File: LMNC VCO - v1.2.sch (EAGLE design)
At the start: 79 parts, among them IC1 CEM3340, J1 JACKS, J10 LINK, J13 OCT SEL, P1 POWER, U1 TL072CP, U2 TL074CN, U4 LM4040AIZ, U5 L7805

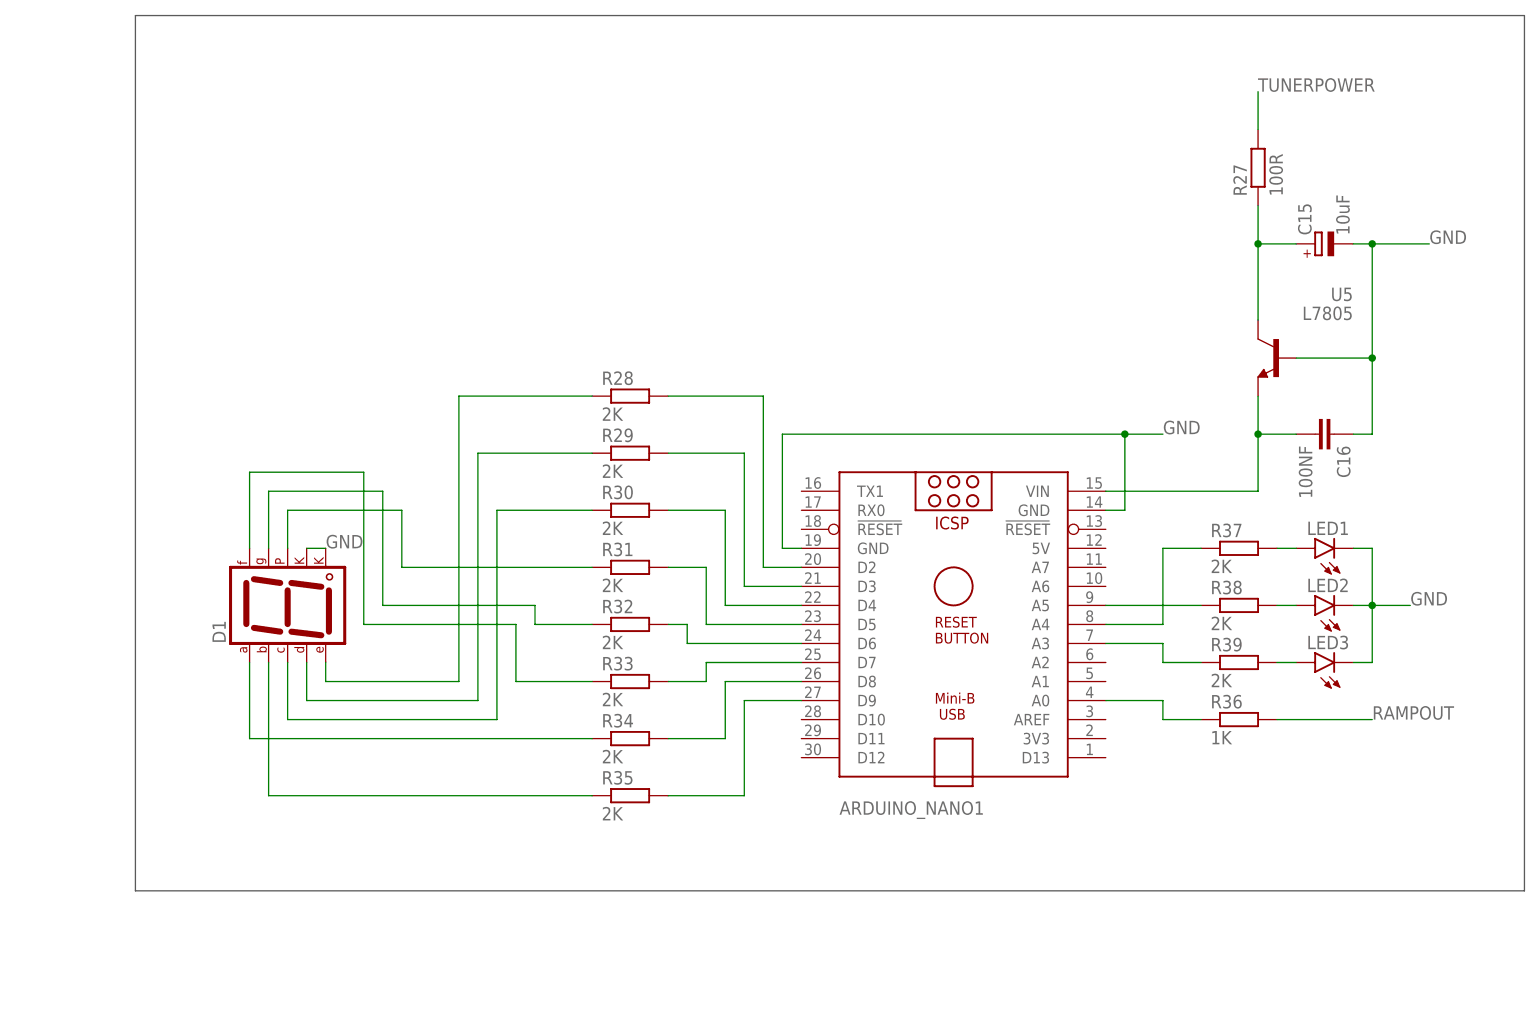
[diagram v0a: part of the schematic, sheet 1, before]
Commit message: Update1
Removed Tuner Arduino,
Replaced Caps to SMD footprint
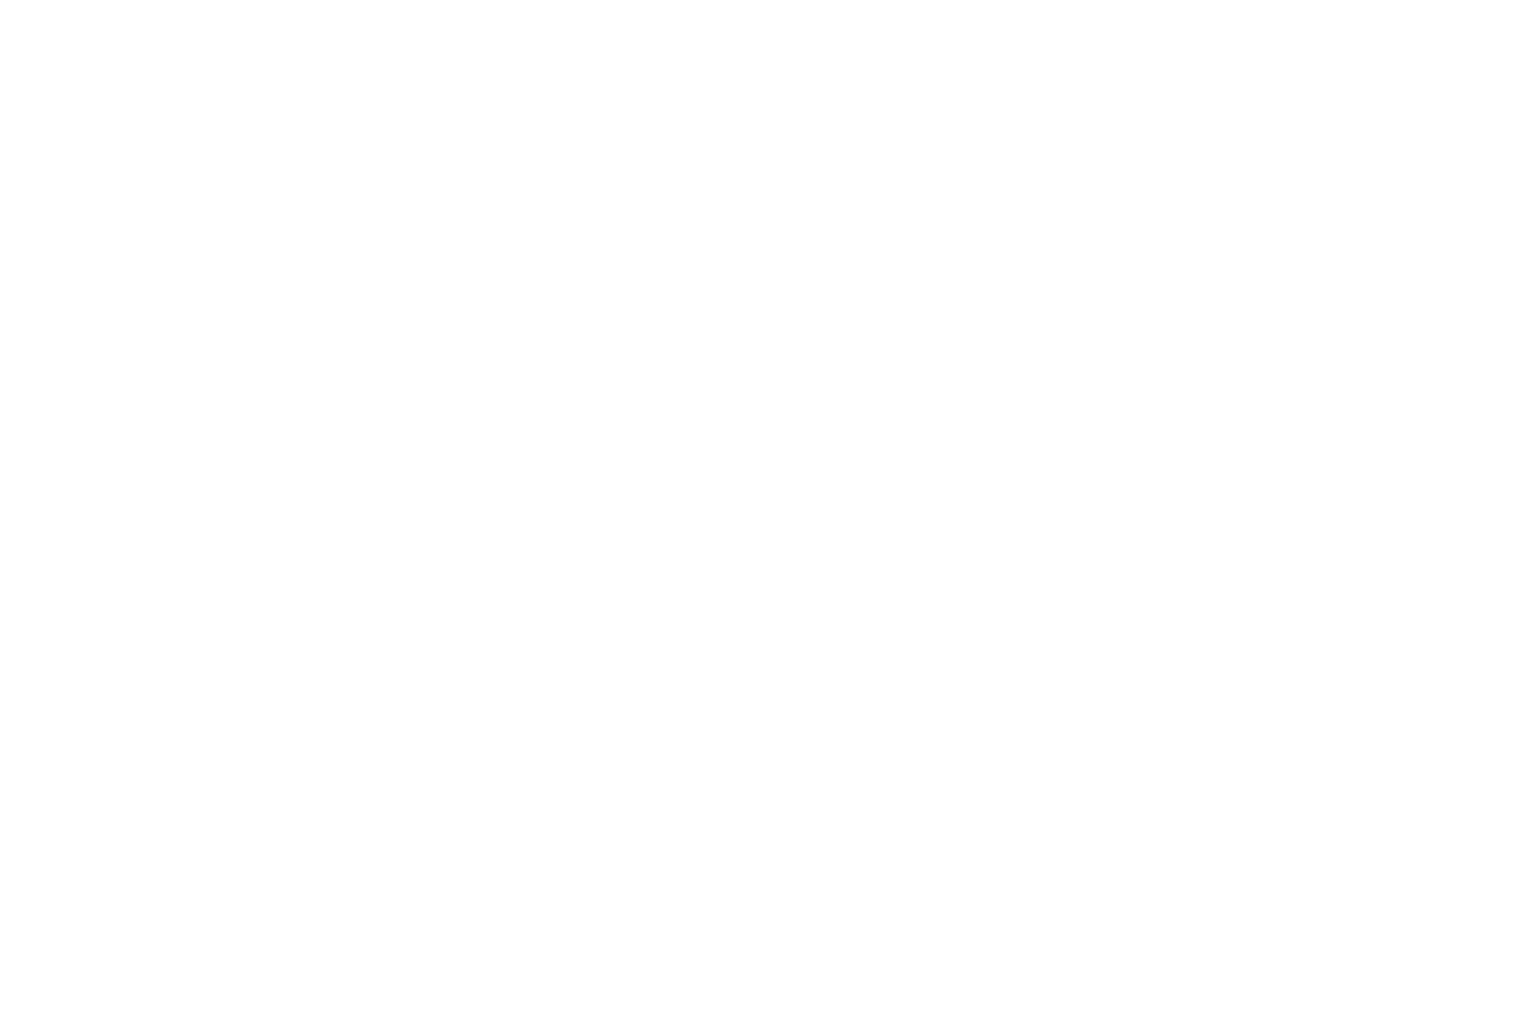
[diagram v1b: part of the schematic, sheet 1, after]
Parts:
- removed ARDUINO_NANO1: (no value), ArduinoNanoV30:ARDUINO_NANO
- removed C15: 10uF, rcl:CPOL-EUE2.5-5
- removed C16: 100NF, capacitor-wima:C2,5-3
- removed D1: (no value), special:7SEG-CK
- removed LED1, LED2, LED3: (no value), led:LED3MM
- removed R27: 100R, rcl:R-EU_0207/10
- removed R28, R29, R30, R31, R32, R33, R34, R35, R37, R38, R39: 2K, rcl:R-EU_0207/10
- removed R36: 1K, rcl:R-EU_0207/10
- removed U5: L7805, transistor:2SC1306
- C1, C10, C11, C12, C2, C3, C4, C5, C6, C7: device capacitor-wima:C2,5-3 -> rcl:C-EUC0603
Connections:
- removed net N$19: C15.+, R27.1, U5.C
- removed net N$25: ARDUINO_NANO1.D6, R32.2
- removed net N$32: ARDUINO_NANO1.D7, R33.2
- removed net N$33: ARDUINO_NANO1.D8, R34.2
- removed net N$34: ARDUINO_NANO1.D9, R35.2
- removed net N$35: ARDUINO_NANO1.D5, R31.2
- removed net N$36: ARDUINO_NANO1.D4, R30.2
- removed net N$37: ARDUINO_NANO1.D3, R29.2
- removed net N$38: ARDUINO_NANO1.D2, R28.2
- removed net N$39: ARDUINO_NANO1.A5, R38.1
- removed net N$40: ARDUINO_NANO1.A3, R39.1
- removed net N$41: ARDUINO_NANO1.A4, R37.1
- removed net N$42: LED1.A, R37.2
- removed net N$43: LED2.A, R38.2
- removed net N$44: LED3.A, R39.2
- removed net N$45: ARDUINO_NANO1.A0, R36.1
- removed net N$46: ARDUINO_NANO1.VIN, C16.2, U5.E
- removed net N$47: D1.B, R35.1
- removed net N$48: D1.A, R34.1
- removed net N$49: D1.C, R30.1
- removed net N$50: D1.D, R29.1
- removed net N$51: D1.E, R28.1
- removed net N$52: D1.F, R33.1
- removed net N$53: D1.G, R32.1
- removed net N$54: D1.DP, R31.1
- net GND: no longer ARDUINO_NANO1.GND@1, ARDUINO_NANO1.GND@2, C15.-, C16.1, D1.CK1, D1.CK2, LED1.C, LED2.C, LED3.C, U5.B
- net RAMPOUT: no longer R36.2
- net TUNERPOWER: no longer R27.2
